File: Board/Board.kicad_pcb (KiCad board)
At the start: 2 copper layers, 75 x 110 mm, 21 parts, among them J1 XT30 Female, U1 BlackPill

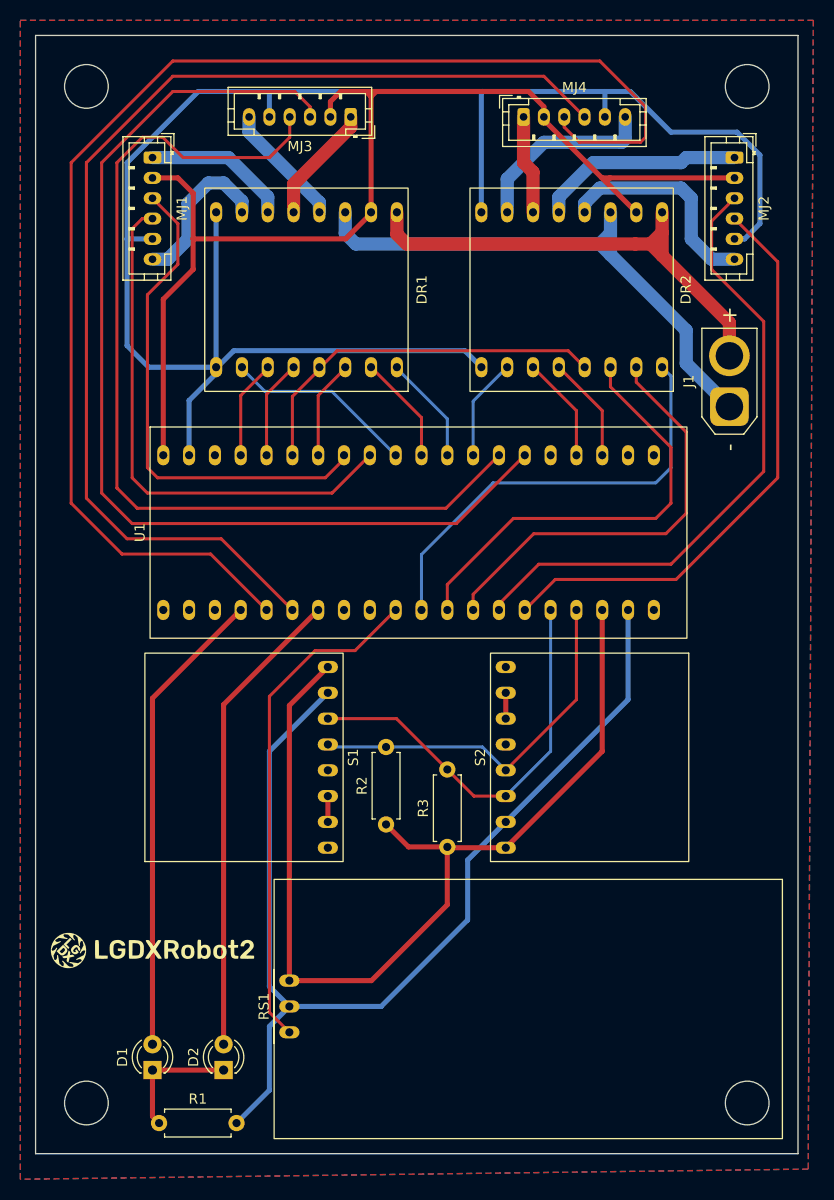
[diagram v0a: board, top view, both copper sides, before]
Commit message: board v2 pcb
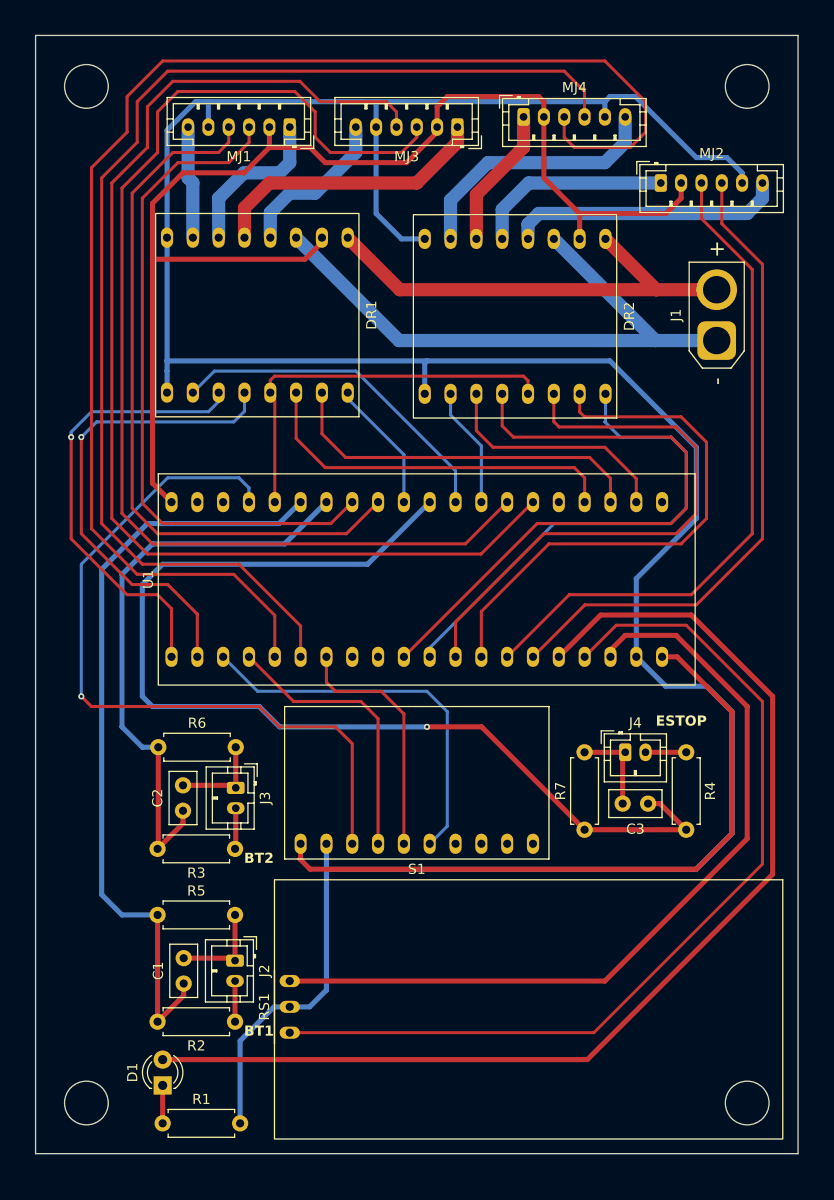
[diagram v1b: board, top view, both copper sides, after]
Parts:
- removed D2: RED_LED, LED_THT:LED_D3.0mm
- removed G***: LOGO, LOGO
- removed S2: INA226, LGDXRobot2:INA226
- added C1: 0.1uF, Capacitor_THT:C_Disc_D5.0mm_W2.5mm_P2.50mm, F.Cu at (112.1, 128.2)
- added C2: 0.1uF, Capacitor_THT:C_Disc_D5.0mm_W2.5mm_P2.50mm, F.Cu at (112.0, 111.2)
- added C3: 0.1uF, Capacitor_THT:C_Disc_D5.0mm_W2.5mm_P2.50mm, F.Cu at (157.8, 110.5)
- added J2: PH2.0 2P, Connector_JST:JST_PH_B2B-PH-K_1x02_P2.00mm_Vertical, F.Cu at (117.1, 126.0)
- added J3: PH2.0 2P, Connector_JST:JST_PH_B2B-PH-K_1x02_P2.00mm_Vertical, F.Cu at (117.2, 109.0)
- added J4: PH2.0 2P, Connector_JST:JST_PH_B2B-PH-K_1x02_P2.00mm_Vertical, F.Cu at (155.5, 105.5)
- added R4: 68k, Resistor_THT:R_Axial_DIN0207_L6.3mm_D2.5mm_P7.62mm_Horizontal, F.Cu at (161.5, 105.5)
- added R5: 10k, Resistor_THT:R_Axial_DIN0207_L6.3mm_D2.5mm_P7.62mm_Horizontal, F.Cu at (109.5, 121.5)
- added R6: 10k, Resistor_THT:R_Axial_DIN0207_L6.3mm_D2.5mm_P7.62mm_Horizontal, F.Cu at (109.6, 105.0)
- added R7: 10k, Resistor_THT:R_Axial_DIN0207_L6.3mm_D2.5mm_P7.62mm_Horizontal, F.Cu at (151.5, 113.1)
- D1: value GREEN_LED -> RED_LED
- R2, R3: value 4k7 -> 68k
- S1: value INA226 -> ~; footprint LGDXRobot2:INA226 -> LGDXRobot2:ICM20948
- moved R2 24.4 mm to (117.1, 132.0), turned to 180 degrees
- moved R3 20.9 mm to (117.1, 115.0), turned to 180 degrees
- moved MJ1 13.8 mm to (122.5, 44.0), turned to 180 degrees
- moved S1 12.2 mm to (135.0, 114.5), turned to 0 degrees
- moved MJ3 10.5 mm to (139.0, 44.0)
- moved MJ2 7.67 mm to (159.0, 49.5), turned to 0 degrees
- moved J1 6.62 mm to (164.5, 65.0)
- moved DR2 6.16 mm to (144.9, 62.6)
- moved DR1 5.44 mm to (119.6, 62.5)
- moved U1 4.68 mm to (135.0, 88.5)
- moved D1 1.81 mm to (110.0, 138.3)
- moved R1 0.35 mm to (110.0, 142.0)
- moved RS1 0.05 mm to (122.5, 130.5)
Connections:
- D1 pad 2: /PB15_D1 -> /PB8_D1
- DR1 pad 15: /PA5_DR1PWMB -> /PA3_DR1PWMB
- DR1 pad 16: /PB10_DR1BIN2 -> /PB12_DR1BIN2
- DR1 pad 17: /PB2_DR1BIN1 -> /PB13_DR1BIN1
- DR1 pad 18: /GND23 -> /GND47
- DR1 pad 19: /PB1_DRxSTBY -> /PB2_DRxSTBY
- DR1 pad 21: /PB0_DR1AIN1 -> /PC15_DR1AIN1
- DR1 pad 22: /PA4_DR1AIN2 -> /PC14_DR1AIN2
- DR1 pad 23: /PA3_DR1PWMA -> /PA5_DR1PWMA
- DR2 pad 16: /PC15_DR2BIN2 -> /PC13_DR2BIN2
- DR2 pad 17: /PC14_DR2BIN1 -> /PA15_DR2BIN1
- DR2 pad 18: /GND23 -> /GND47
- DR2 pad 19: /PB1_DRxSTBY -> /PB2_DRxSTBY
- MJ1 pad 5: /GND23 -> /GND47
- MJ2 pad 5: /GND23 -> /GND47
- MJ3 pad 3: /PA0_MJ3CH2 -> /PA1_MJ3CH2
- MJ3 pad 4: /PA1_MJ3CH1 -> /PA0_MJ3CH1
- MJ3 pad 5: /GND23 -> /GND47
- MJ4 pad 5: /GND23 -> /GND47
- R2 pad 1: /5V99 -> Net-(J2-Pin_2)
- R2 pad 2: /PB9_SDA -> /PB1_BT1
- R3 pad 1: /5V99 -> Net-(J3-Pin_2)
- R3 pad 2: /PB8_SCL -> /PB0_BT2
- RS1 pad 3: /PA15_RS1 -> /PB9_RS1
- S1 pad 3: unconnected-(S1-~{Alert}-Pad3) -> /PB10_SCLK
- S1 pad 4: /PB9_SDA -> /PB15_SDA
- S1 pad 5: /PB8_SCL -> /PA10_NCS
- S1 pad 6: /5V99 -> /PB14_ADO
- S1 pad 7: /GND47 -> unconnected-(S1-INT-Pad7)
- S1 pad 8: /S1Vbus -> unconnected-(S1-FSY-Pad8)
- S1 pad 9: /S1Vbus -> unconnected-(S1-ACL-Pad9)
- U1 pad 10: /PA0_MJ3CH2 -> /PA0_MJ3CH1
- U1 pad 11: /PA1_MJ3CH1 -> /PA1_MJ3CH2
- U1 pad 13: /PA3_DR1PWMA -> /PA3_DR1PWMB
- U1 pad 14: /PA4_DR1AIN2 -> /PA4_ESTOP
- U1 pad 15: /PA5_DR1PWMB -> /PA5_DR1PWMA
- U1 pad 18: /PB0_DR1AIN1 -> /PB0_BT2
- U1 pad 19: /PB1_DRxSTBY -> /PB1_BT1
- U1 pad 2: unconnected-(U1-PC13-Pad2) -> /PC13_DR2BIN2
- U1 pad 20: /PB2_DR1BIN1 -> /PB2_DRxSTBY
- U1 pad 21: /PB10_DR1BIN2 -> /PB10_SCLK
- U1 pad 23: /GND23 -> unconnected-(U1-GND-Pad23)
- U1 pad 25: unconnected-(U1-PB12-Pad25) -> /PB12_DR1BIN2
- U1 pad 26: unconnected-(U1-PB13-Pad26) -> /PB13_DR1BIN1
- U1 pad 27: unconnected-(U1-PB14-Pad27) -> /PB14_ADO
- U1 pad 28: /PB15_D1 -> /PB15_SDA
- U1 pad 3: /PC14_DR2BIN1 -> /PC14_DR1AIN2
- U1 pad 31: /PA10_D2 -> /PA10_NCS
- U1 pad 38: /PA15_RS1 -> /PA15_DR2BIN1
- U1 pad 4: /PC15_DR2BIN2 -> /PC15_DR1AIN1
- U1 pad 45: /PB8_SCL -> /PB8_D1
- U1 pad 46: /PB9_SDA -> /PB9_RS1
- U1 pad 48: unconnected-(U1-3V3-Pad48) -> /3V348
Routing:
- net /GND47: track 105.8 -> 288.7 mm
- net /GND23: track 177.6 -> 0.00 mm
- net /PA0_MJ3CH1: track 0.00 -> 115.2 mm
- net /PA1_MJ3CH2: track 0.00 -> 113.7 mm
- net /PB8_D1: track 0.00 -> 111.1 mm
- net /PA4_ESTOP: track 0.00 -> 106.5 mm, vias 0 -> 1
- net /PA0_MJ3CH2: track 103.2 -> 0.00 mm
- net /PA1_MJ3CH1: track 94.3 -> 0.00 mm
- net /PB9_RS1: track 0.00 -> 91.3 mm
- net /PB1_BT1: track 0.00 -> 75.5 mm
- net /PB10_SCLK: track 0.00 -> 73.2 mm, vias 0 -> 1
- net /3V348: track 0.00 -> 67.0 mm
- net /PA15_DR2BIN1: track 0.00 -> 61.7 mm
- net /PB0_BT2: track 0.00 -> 57.3 mm
- net /PA15_RS1: track 49.8 -> 0.00 mm
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- removed copper zone on B.Cu, net /GND47
- removed copper zone on F.Cu, net /GND47
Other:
- board text added: "BT1"
- board text added: "BT2"
- board text added: "ESTOP"
